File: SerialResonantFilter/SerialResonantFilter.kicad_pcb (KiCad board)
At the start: 2 copper layers, 30.5 x 25.9 mm, 11 parts, among them J1 OUT, J2 INP

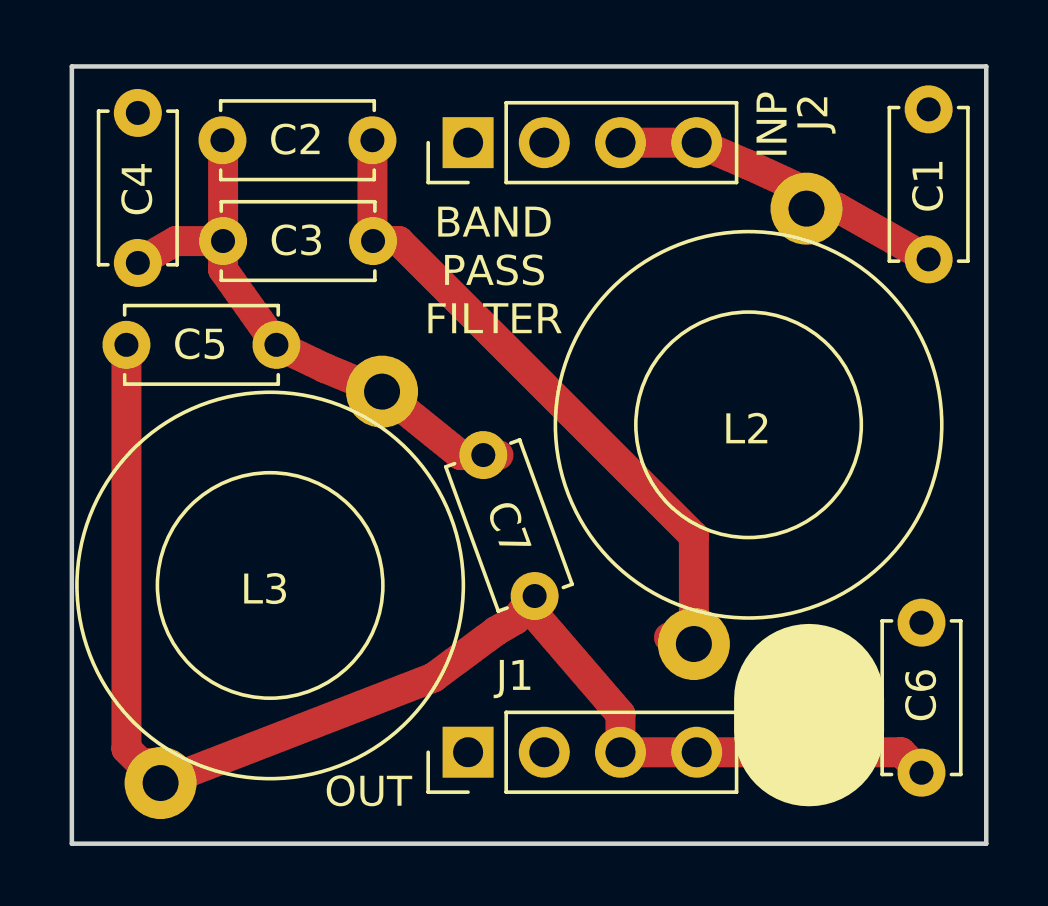
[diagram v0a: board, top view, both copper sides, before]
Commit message: Converted all Kicad projects to version 6.0.10
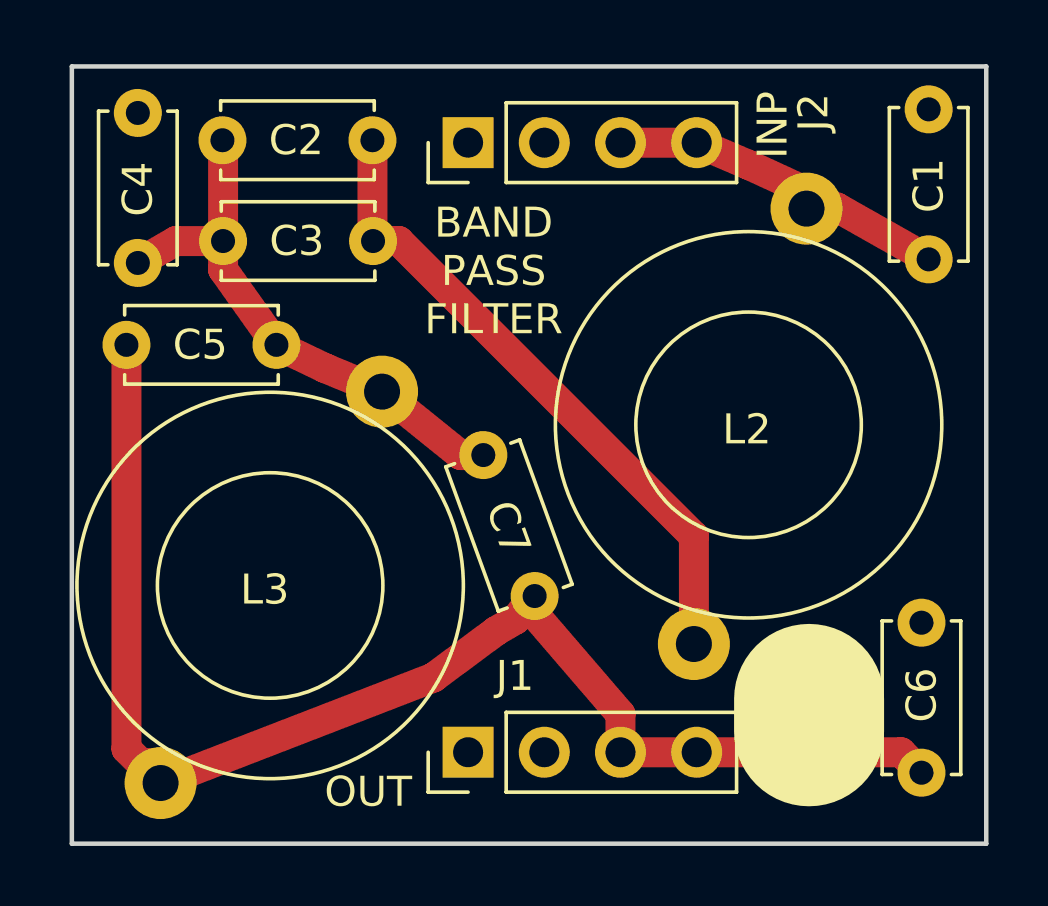
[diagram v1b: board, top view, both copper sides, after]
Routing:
- net Net-(C3-Pad1): track 22.5 -> 21.7 mm
- net Net-(C2-Pad2): track 19.1 -> 18.5 mm
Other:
- net class Default removed

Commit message: Made capacitors on board dual footprint
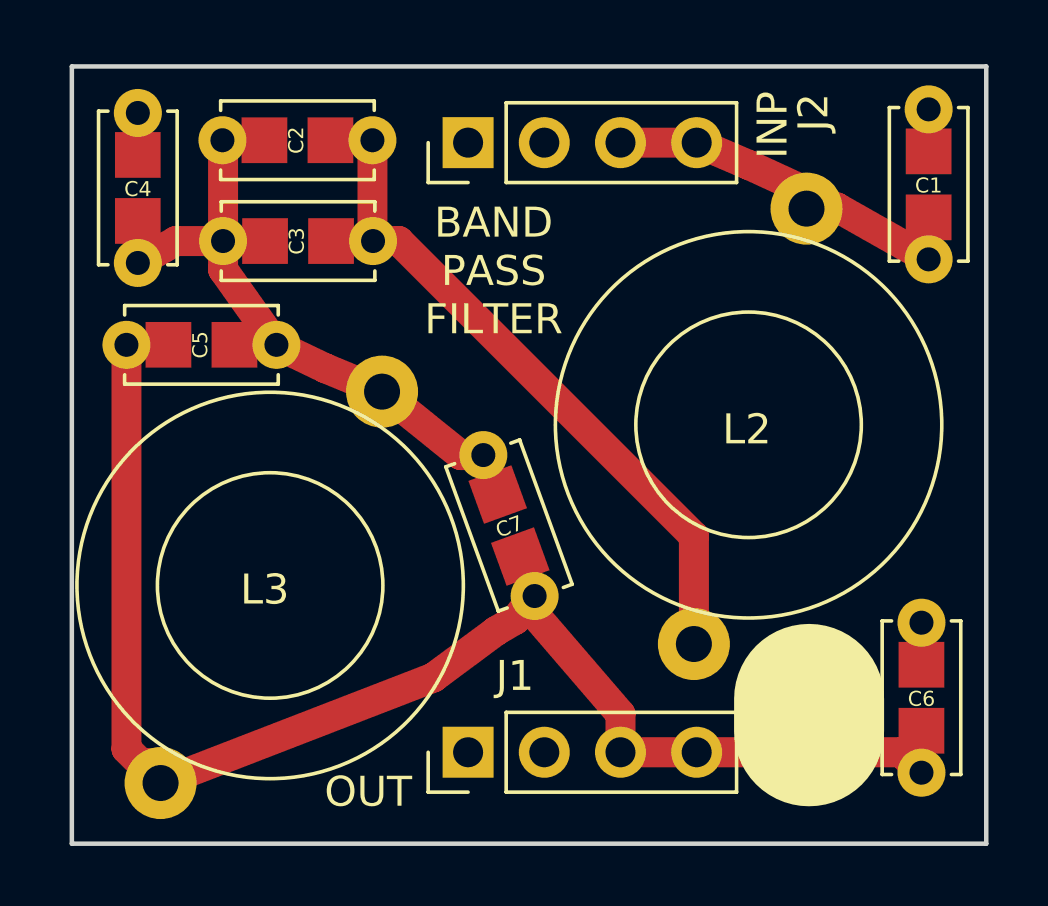
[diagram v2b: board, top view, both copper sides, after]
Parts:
- C1, C2, C3, C4, C5, C6, C7: footprint Capacitors_THT:C_Disc_D5.0mm_W2.5mm_P5.00mm -> SerialResonantFilter:C_Disc_D5.0mm_W2.5mm_P5.00mm_Dual

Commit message: Changed size of text on capacitor footprint
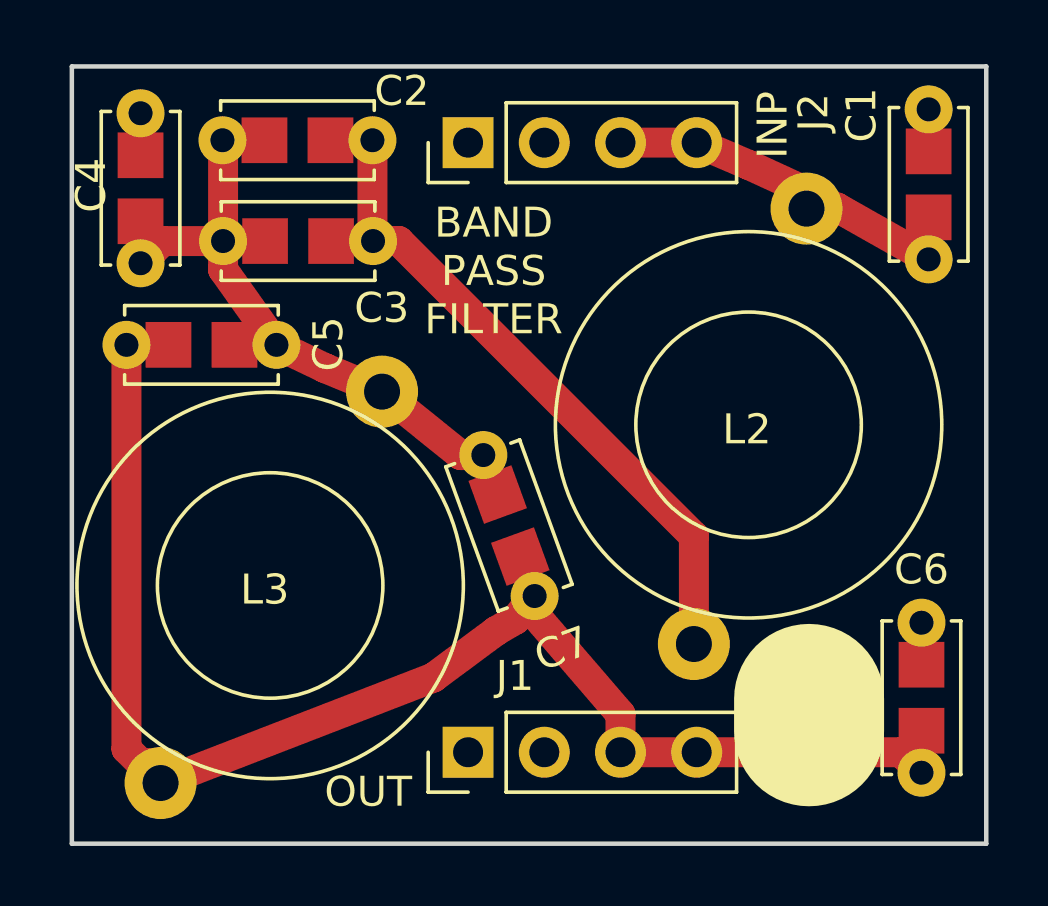
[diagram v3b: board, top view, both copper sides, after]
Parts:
- moved C4 0.09 mm to (121.7, 90.5)
